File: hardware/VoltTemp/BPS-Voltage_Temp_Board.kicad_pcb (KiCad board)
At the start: 2 copper layers, 98.2 x 56.2 mm, 138 parts, among them IC1 ISO1641BDR, J10 53307-2471, J11 Conn_01x07, J12 Conn_01x04, J13 Conn_01x04, J5 Logic_Analyzer, J6 Conn_01x04, J7 Conn_01x04, J8 Conn_01x06, J9 Conn_01x03, SW1 BOOT, U1 EL3H7, U12 TLV9062xD, U13 TLV9062xD, U14 TLV9062xD, U2 BQ7692003PW, U3 EL3H7, U4 TLV9062xD, U6 TLV9062xD

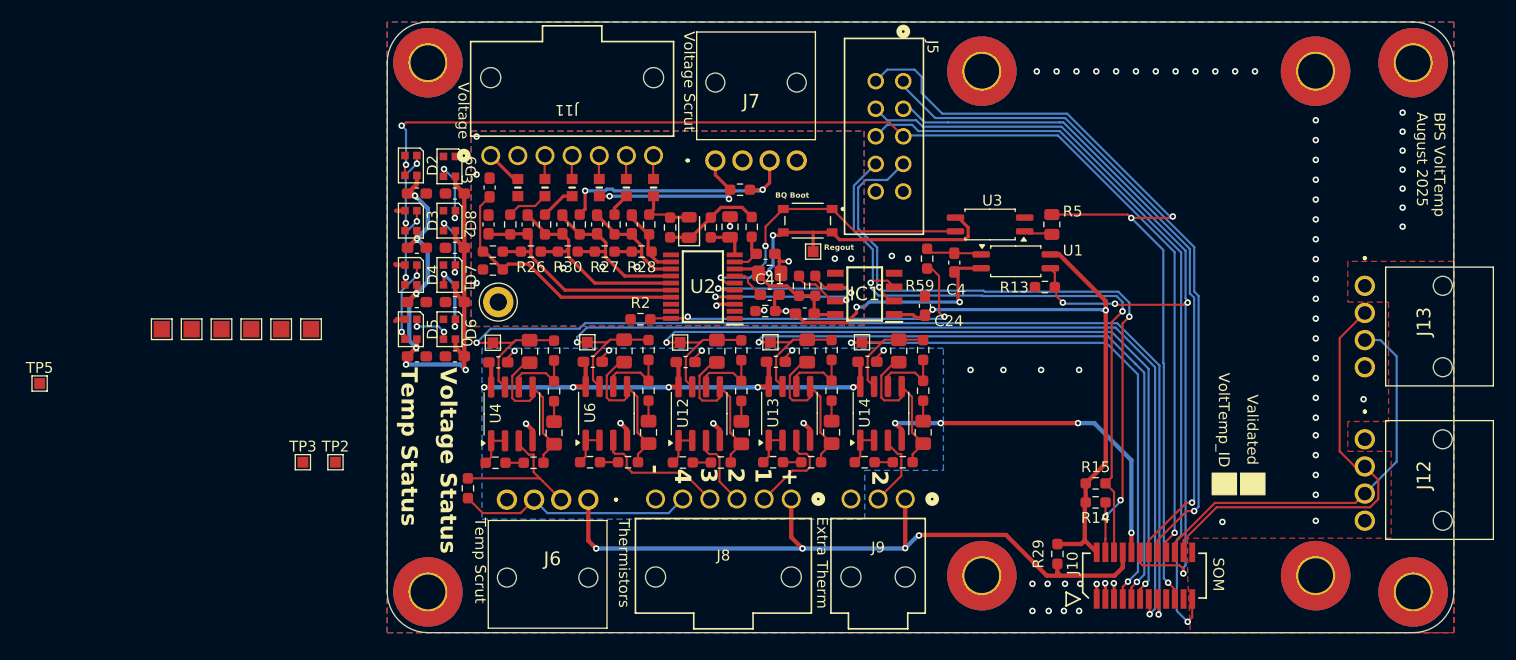
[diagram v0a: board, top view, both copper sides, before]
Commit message: redid thermistor board
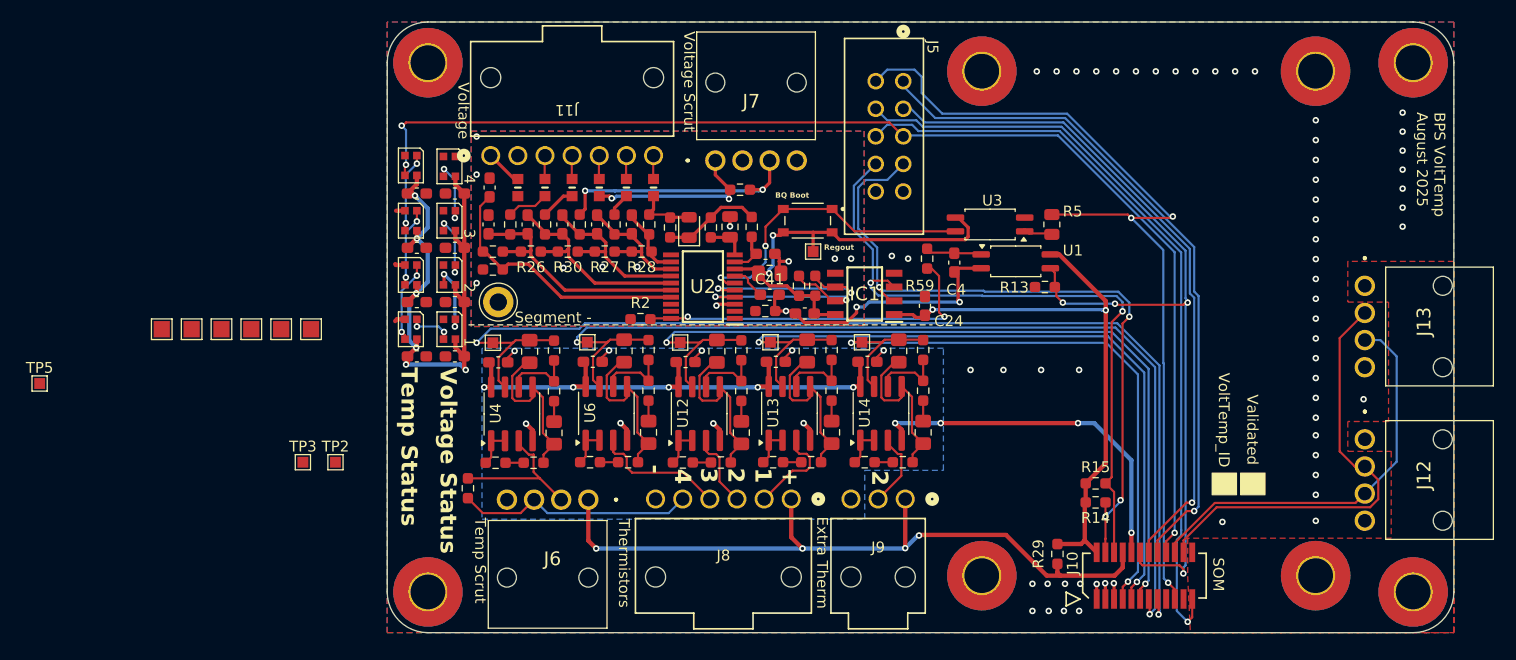
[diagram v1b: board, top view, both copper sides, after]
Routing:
- net /VoltageSense/bmsBoot: track 29.3 -> 28.5 mm, vias 3 -> 2
- net /TemperatureConn/rawTemperature4: track 14.4 -> 13.9 mm
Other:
- board text added: "Segment -"
- board text removed: "0"
